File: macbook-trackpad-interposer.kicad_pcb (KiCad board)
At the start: 2 copper layers, 36.8 x 12.7 mm, 28 parts, among them CN1 DF40C-50DP-0.4V(51), CN2 DF40C-50DS-0.4V(51)

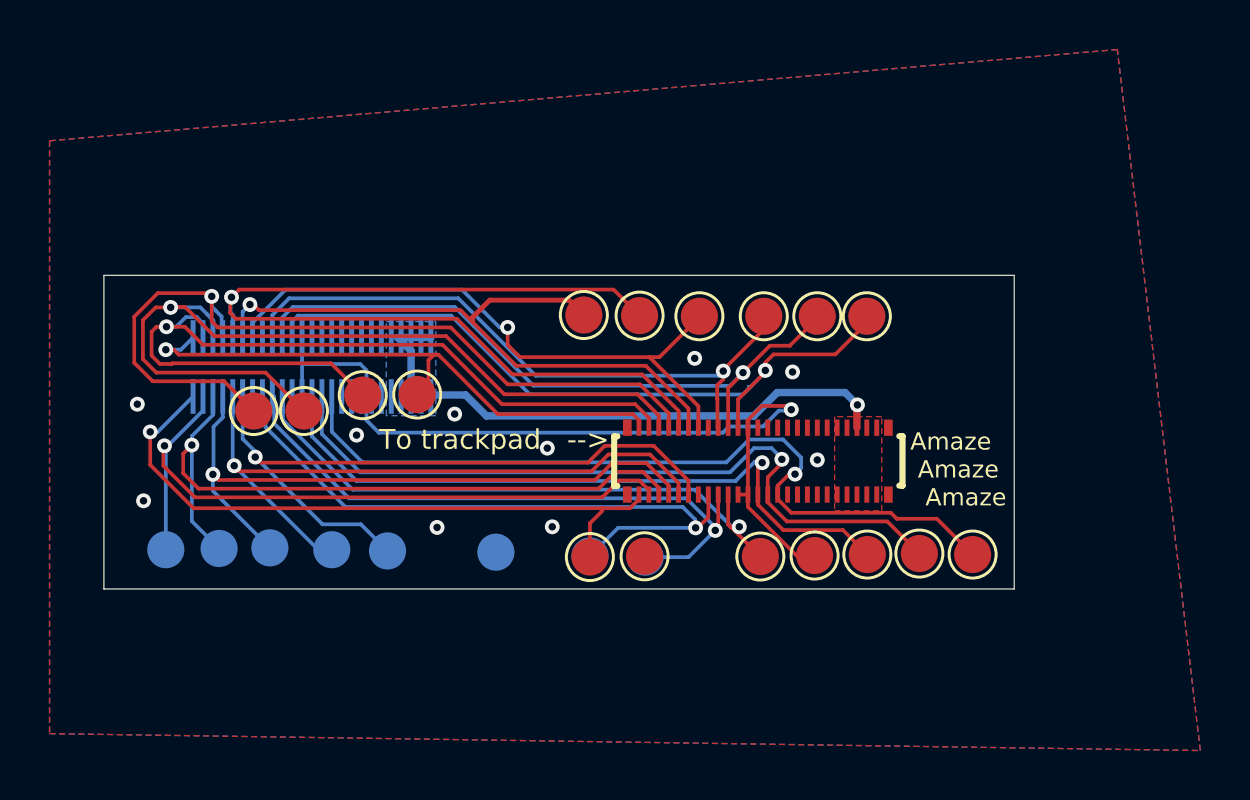
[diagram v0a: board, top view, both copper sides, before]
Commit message: unfuck the pcb
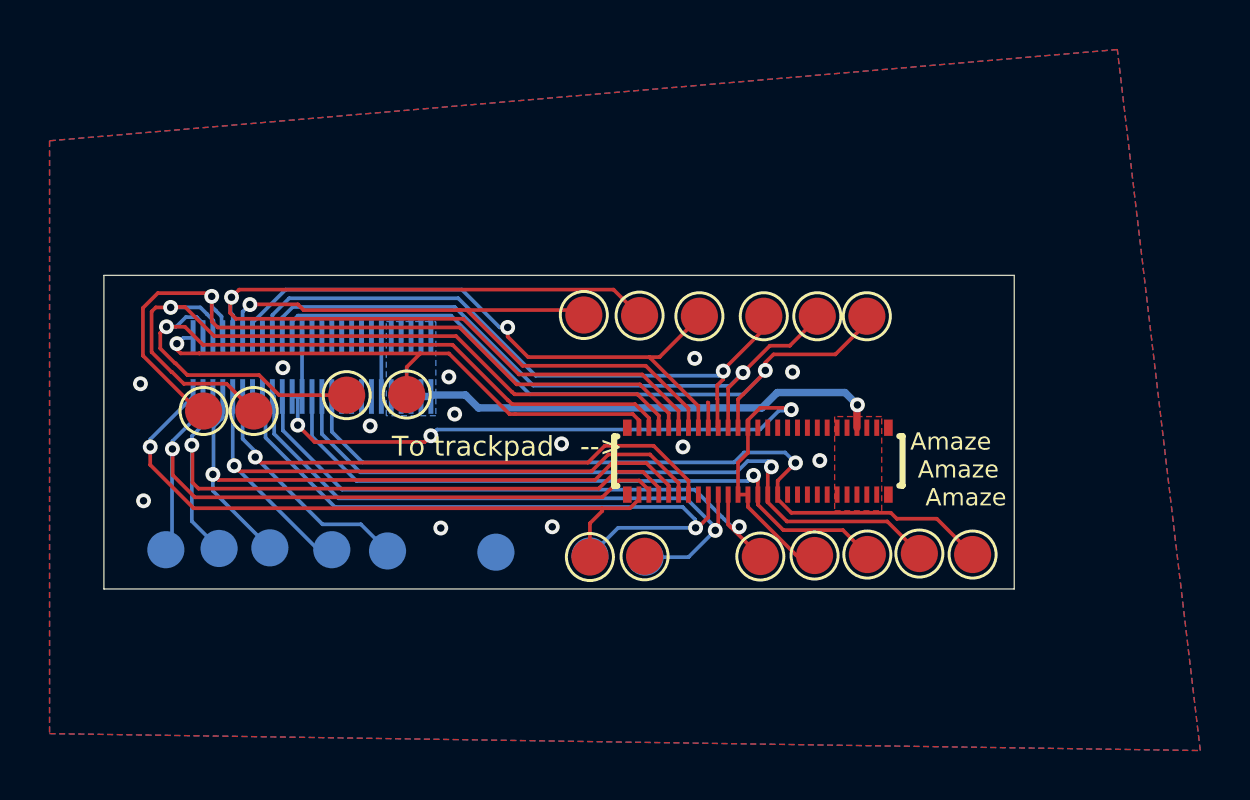
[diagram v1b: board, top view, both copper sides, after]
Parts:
- moved TP3 2.03 mm to (134.8, 75.8)
- moved TP4 2.03 mm to (132.7, 75.8)
- moved TP2 0.65 mm to (138.5, 75.1)
- moved TP1 0.42 mm to (140.9, 75.1)
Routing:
- net PPBUS_AON: track 23.9 -> 20.3 mm
- net GND: track 0.00 -> 3.42 mm, vias 10 -> 13
- net /I2C_KBD_SDA: track 34.5 -> 31.8 mm
- net /I2C_KBD_SCL: track 34.9 -> 32.2 mm
- net /I2C_TPAD_CONN_SCL: track 35.2 -> 33.6 mm
- net /SWD_IPD_DATA_CONN: track 28.0 -> 26.8 mm
- net /SWD_IPD_CLK_CONN: track 30.3 -> 29.1 mm
- net /IPD_MTP_FUNC_1_CONN: track 32.6 -> 31.6 mm
- net /I2C_TPAD_CONN_SDA: track 24.0 -> 23.0 mm
- net /PP3V3_S2_HOLD_IPD: track 34.7 -> 34.2 mm, vias 1 -> 3
